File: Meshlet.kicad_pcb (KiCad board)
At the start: 4 copper layers, 42.5 x 32 mm, 101 parts, among them J12 GPS Header, J13 Thermistor Pins, J14 Ext. Notif. Header, J2 User Btn Header, J3 Batt. Header (Picoblade 1.25), J4 Batt. Header (JST-PH 2.0), J5 USB_C_Receptacle_USB2.0_16P, J6 I2C Header, J7 Ext. Power Header, J9 Ext. Power Header, Q1 AO3400A, SW2 BOOTSEL, U1 XC6206PxxxMR, U11 INA3221, U2 USBLC6-2SC6, U3 XC6206PxxxMR, U4 RP2350_60QFN, U5 Wio-SX1262, U6 BQ25185, U7 BME280, U8 W25Q32JVZP, U9 XC6206PxxxMR, Y1 12.000MHz

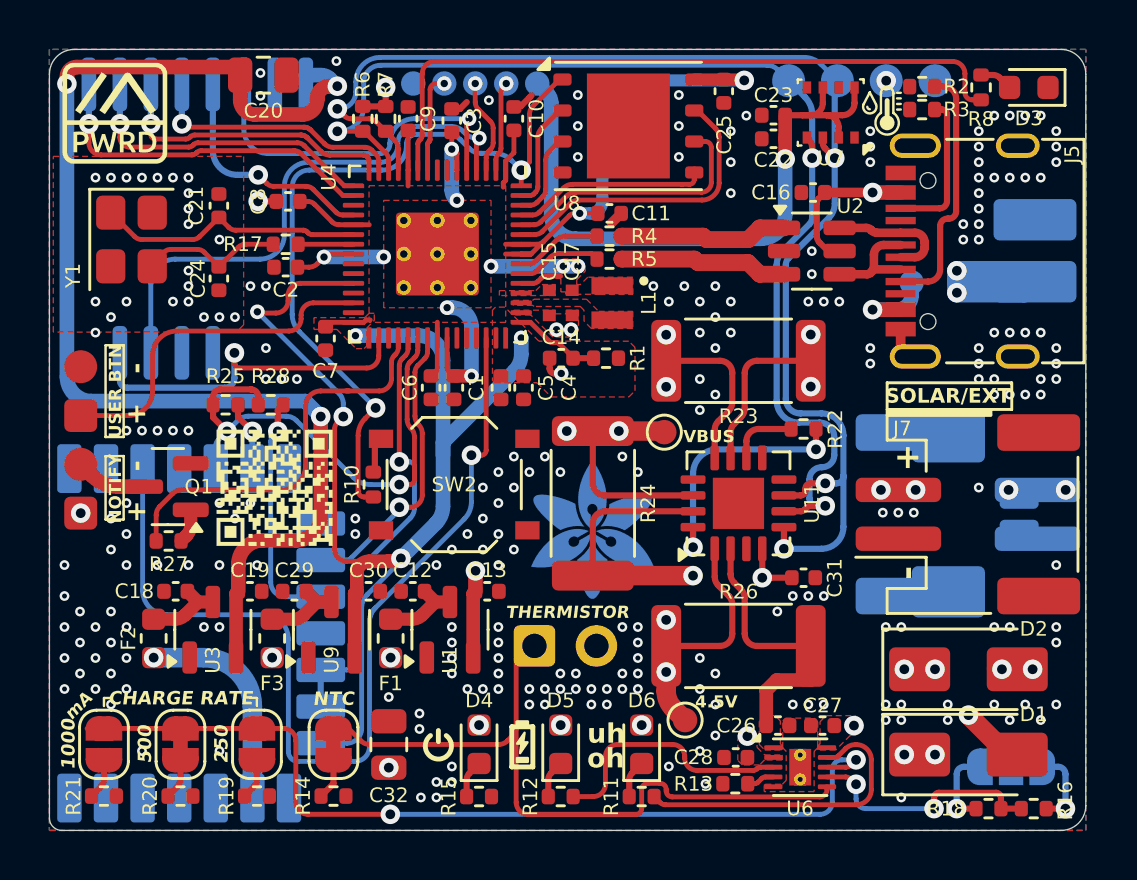
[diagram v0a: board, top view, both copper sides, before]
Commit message: Just in case commit before changing via stitching
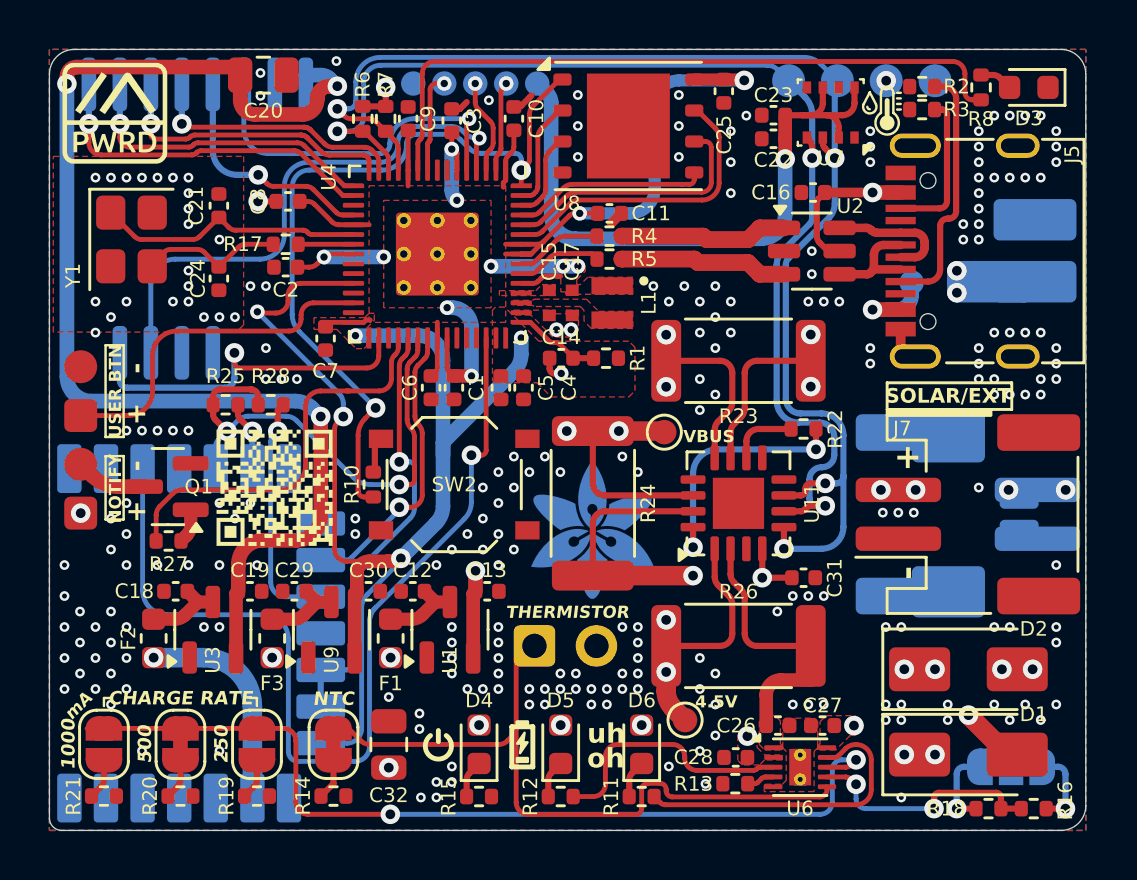
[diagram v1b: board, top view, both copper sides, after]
